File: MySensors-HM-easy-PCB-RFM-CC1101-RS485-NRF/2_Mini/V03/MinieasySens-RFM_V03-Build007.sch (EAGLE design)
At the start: 29 parts, among them IC1 ATSHA204A, IC2 REG1117, IC3 LD117ADT50TR, IC4 LM1117MPX-ADJ, M1 ARDUINO-PRO-MINI-3.3V#NP, U1 RFM69HCW

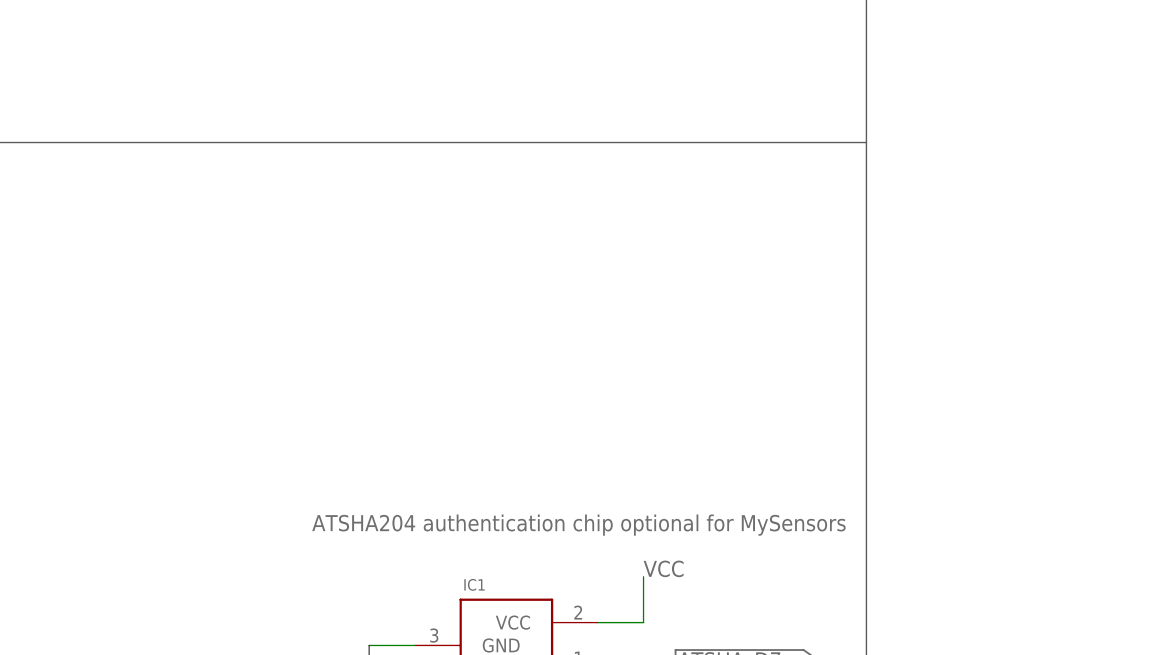
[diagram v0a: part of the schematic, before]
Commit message: V03
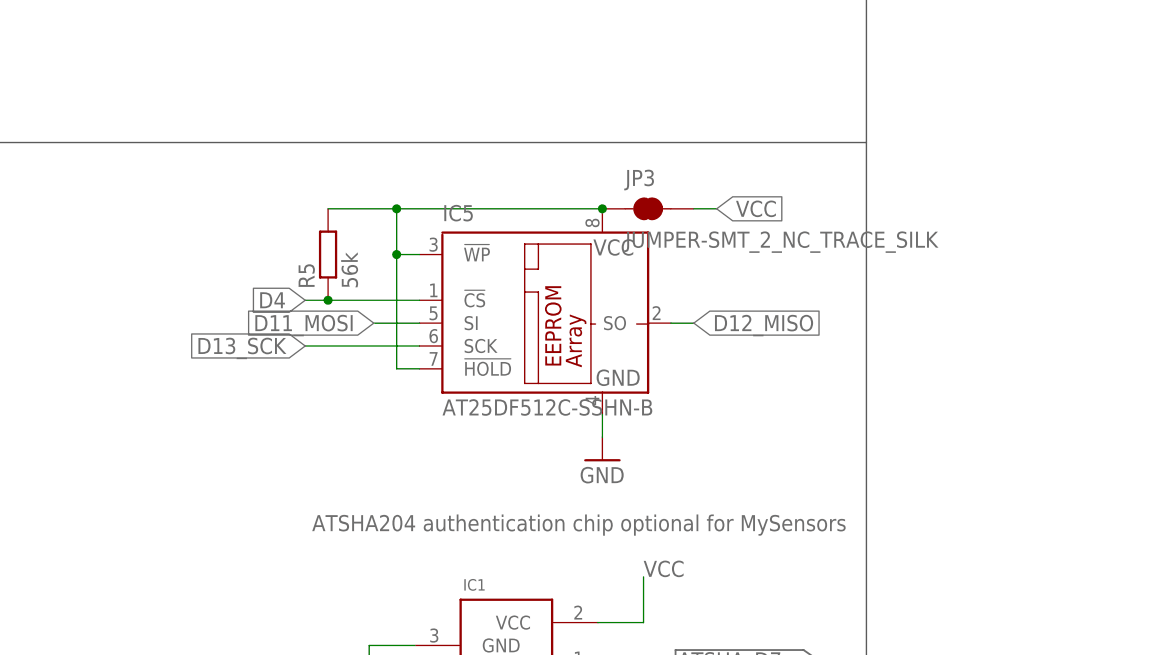
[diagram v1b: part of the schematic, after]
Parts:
- added IC5: AT25DF512C-SSHN-B, microchip:25AA080SN
- added JP3: JUMPER-SMT_2_NC_TRACE_SILK, SparkFun-Jumpers:JUMPER-SMT_2_NC_TRACE_SILK
- added R5: 56k, resistor:R-EU_M0805
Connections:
- new net VCC1: IC5.!HOLD, IC5.!WP, IC5.VCC, JP3.1, R5.2
- net D11_MOSI: now also IC5.SI
- net D12_MISO: now also IC5.SO
- net D13_SCK: now also IC5.SCK
- net D4: now also IC5.!CS, R5.1
- net GND: now also IC5.GND
- net VCC: now also JP3.2
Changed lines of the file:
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@@
 <part name="U1" library="doug" deviceset="RFM69H" device="CW"/>
 <part name="ANT2" library="pinhead" deviceset="PINHD-1X1" device=""/>
+<part name="IC5" library="microchip" deviceset="25*" device="SN" technology="AA080" value="AT25DF512C-SSHN-B"/>
+<part name="GND2" library="supply1" deviceset="GND" device=""/>
+<part name="R5" library="resistor" deviceset="R-EU_" device="M0805" value="56k"/>
+<part name="JP3" library="SparkFun-Jumpers" deviceset="JUMPER-SMT_2_NC_TRACE" device="_SILK"/>
 </parts>
 <sheets>
@@
 <attribute name="VALUE" x="87.63" y="99.06" size="1.778" layer="96"/>
 </instance>
+<instance part="IC5" gate="G$1" x="124.968" y="53.594" smashed="yes">
+<attribute name="NAME" x="114.808" y="64.924" size="1.778" layer="95"/>
+<attribute name="VALUE" x="114.808" y="43.334" size="1.778" layer="96"/>
+</instance>
+<instance part="GND2" gate="1" x="132.588" y="38.354" smashed="yes">
+<attribute name="VALUE" x="130.048" y="35.814" size="1.778" layer="96"/>
+</instance>
+<instance part="R5" gate="G$1" x="102.108" y="61.214" smashed="yes" rot="R90">
+<attribute name="NAME" x="100.6094" y="57.404" size="1.778" layer="95" rot="R90"/>
+<attribute name="VALUE" x="105.41" y="57.404" size="1.778" layer="96" rot="R90"/>
+</instance>
+<instance part="JP3" gate="G$1" x="137.668" y="66.294" smashed="yes">
+<attribute name="NAME" x="135.128" y="68.834" size="1.778" layer="95" font="vector"/>
+<attribute name="VALUE" x="135.128" y="63.754" size="1.778" layer="96" font="vector" align="top-left"/>
+</instance>
 </instances>
 <busses>
@@
 <wire x1="-58.42" y1="96.52" x2="-58.42" y2="83.82" width="0.1524" layer="91"/>
 <label x="-58.42" y="83.82" size="1.778" layer="95" rot="R270" xref="yes"/>
+</segment>
+<segment>
+<pinref part="GND2" gate="1" pin="GND"/>
+<pinref part="IC5" gate="G$1" pin="GND"/>
+<wire x1="132.588" y1="40.894" x2="132.588" y2="43.434" width="0.1524" layer="91"/>
 </segment>
 </net>
@@
 <label x="-63.5" y="83.82" size="1.778" layer="95" rot="R270" xref="yes"/>
 </segment>
+<segment>
+<pinref part="JP3" gate="G$1" pin="2"/>
+<wire x1="142.748" y1="66.294" x2="145.288" y2="66.294" width="0.1524" layer="91"/>
+<label x="145.288" y="66.294" size="1.778" layer="95" xref="yes"/>
+</segment>
 </net>
 <net name="A4" class="0">
@@
 <label x="12.7" y="12.7" size="1.778" layer="95" rot="R270" xref="yes"/>
 </segment>
+<segment>
+<pinref part="IC5" gate="G$1" pin="!CS"/>
+<wire x1="112.268" y1="56.134" x2="102.108" y2="56.134" width="0.1524" layer="91"/>
+<label x="99.568" y="56.134" size="1.778" layer="95" rot="R180" xref="yes"/>
+<pinref part="R5" gate="G$1" pin="1"/>
+<wire x1="102.108" y1="56.134" x2="99.568" y2="56.134" width="0.1524" layer="91"/>
+<junction x="102.108" y="56.134"/>
+</segment>
 </net>
 <net name="D3" class="0">
@@
 <label x="73.66" y="190.5" size="1.778" layer="95"/>
 </segment>
+<segment>
+<pinref part="IC5" gate="G$1" pin="SI"/>
+<wire x1="112.268" y1="53.594" x2="107.188" y2="53.594" width="0.1524" layer="91"/>
+<label x="107.188" y="53.594" size="1.778" layer="95" rot="R180" xref="yes"/>
+</segment>
 </net>
 <net name="D12_MISO" class="0">
@@
 <label x="73.66" y="185.42" size="1.778" layer="95"/>
 </segment>
+<segment>
+<pinref part="IC5" gate="G$1" pin="SO"/>
+<wire x1="140.208" y1="53.594" x2="142.748" y2="53.594" width="0.1524" layer="91"/>
+<label x="142.748" y="53.594" size="1.778" layer="95" xref="yes"/>
+</segment>
 </net>
 <net name="D13_SCK" class="0">
@@
 <wire x1="71.12" y1="180.34" x2="88.9" y2="180.34" width="0.1524" layer="91"/>
 <label x="73.66" y="180.34" size="1.778" layer="95"/>
+</segment>
+<segment>
+<pinref part="IC5" gate="G$1" pin="SCK"/>
+<wire x1="112.268" y1="51.054" x2="99.568" y2="51.054" width="0.1524" layer="91"/>
+<label x="99.568" y="51.054" size="1.778" layer="95" rot="R180" xref="yes"/>
 </segment>
 </net>
@@
 </segment>
 </net>
+<net name="VCC1" class="1">
+<segment>
+<pinref part="IC5" gate="G$1" pin="!HOLD"/>
+<wire x1="112.268" y1="48.514" x2="109.728" y2="48.514" width="0.1524" layer="91"/>
+<wire x1="109.728" y1="48.514" x2="109.728" y2="61.214" width="0.1524" layer="91"/>
+<pinref part="IC5" gate="G$1" pin="!WP"/>
+<wire x1="109.728" y1="61.214" x2="112.268" y2="61.214" width="0.1524" layer="91"/>
+<pinref part="IC5" gate="G$1" pin="VCC"/>
+<wire x1="132.588" y1="66.294" x2="109.728" y2="66.294" width="0.1524" layer="91"/>
+<wire x1="109.728" y1="66.294" x2="109.728" y2="61.214" width="0.1524" layer="91"/>
+<junction x="109.728" y="61.214"/>
+<junction x="109.728" y="66.294"/>
+<wire x1="102.108" y1="66.294" x2="109.728" y2="66.294" width="0.1524" layer="91"/>
+<pinref part="R5" gate="G$1" pin="2"/>
+<pinref part="JP3" gate="G$1" pin="1"/>
+<junction x="132.588" y="66.294"/>
+</segment>
+</net>
